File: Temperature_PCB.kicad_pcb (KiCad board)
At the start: 2 copper layers, 29 parts, among them K1 HF115F/024-1H3B, Q1 2N7002, U2 LM393, U5 AMS1117-5.0

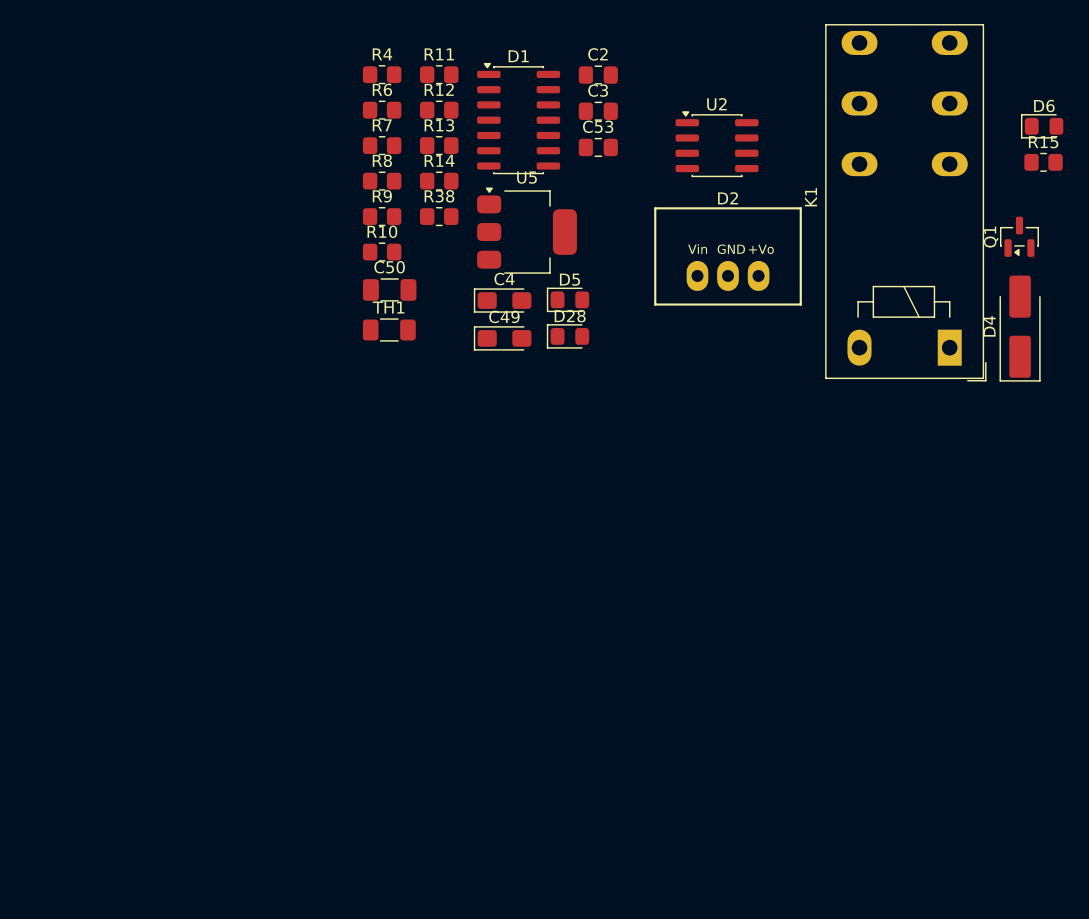
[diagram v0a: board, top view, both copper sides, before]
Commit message: VER1.0: плата разведена, файлы для производства готовы
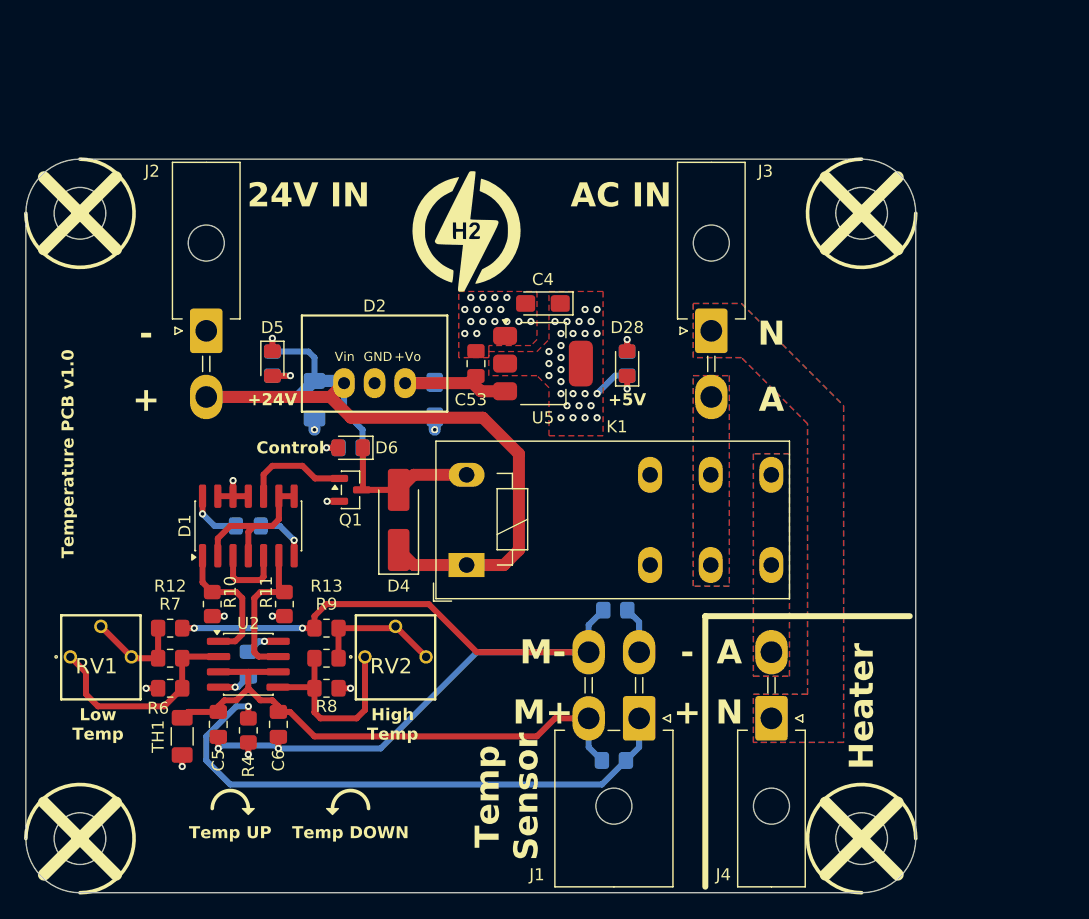
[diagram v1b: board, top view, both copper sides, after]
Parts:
- added C5: 100n, Capacitor_SMD:C_0805_2012Metric_Pad1.18x1.45mm_HandSolder, F.Cu at (127.5, 141.5)
- added C6: 100n, Capacitor_SMD:C_0805_2012Metric_Pad1.18x1.45mm_HandSolder, F.Cu at (132.5, 141.5)
- added D3: Logo, Logo_My:Logo_Company_2, F.Cu at (148.1, 100.5)
- added H1: MountingHole, MountingHole:MountingHole_4.3mm_M4, F.Cu at (181.0, 99.0)
- added H2: MountingHole, MountingHole:MountingHole_4.3mm_M4, F.Cu at (116.0, 99.0)
- added H3: MountingHole, MountingHole:MountingHole_4.3mm_M4, F.Cu at (181.0, 151.0)
- added H4: MountingHole, MountingHole:MountingHole_4.3mm_M4, F.Cu at (116.0, 151.0)
- added J1: ~, Connector_Molex:Molex_Mini-Fit_Jr_5569-04A2_2x02_P4.20mm_Horizontal, F.Cu at (162.5, 141.0)
- added J2: ~, Connector_Molex:Molex_Mini-Fit_Jr_5569-02A2_2x01_P4.20mm_Horizontal, F.Cu at (126.5, 108.8)
- added J3: ~, Connector_Molex:Molex_Mini-Fit_Jr_5569-02A2_2x01_P4.20mm_Horizontal, F.Cu at (168.5, 108.8)
- added J4: ~, Connector_Molex:Molex_Mini-Fit_Jr_5569-02A2_2x01_P4.20mm_Horizontal, F.Cu at (173.5, 141.0)
- added R16: 0, Resistor_SMD:R_0805_2012Metric_Pad1.20x1.40mm_HandSolder, B.Cu at (160.5, 132.0)
- added R5: 0, Resistor_SMD:R_0805_2012Metric_Pad1.20x1.40mm_HandSolder, B.Cu at (160.4, 144.5)
- added RV1: ~, Potentiometer_my:3362P_1, F.Cu at (117.7, 139.4)
- added RV2: ~, Potentiometer_my:3362P_1, F.Cu at (142.2, 139.4)
- C2, C3, C49, C50, R14, R15, R38: moved to B.Cu
- D1: value CD4011 -> ~
- D2: value K7809-500R3 -> ~
- D4: value 1N4007[M7] -> ~
- K1: value HF115F/024-1H3B -> ~
- Q1: value 2N7002 -> ~
- R7: value 20 -> 49.9
- R9: value 49.9 -> 330
- TH1: value Thermistor_NTC_3Wire -> Thermistor_NTC
- U2: value LM393 -> ~
- U5: value AMS1117-5.0 -> ~
- moved D6 63.6 mm to (138.5, 118.5), turned to 180 degrees
- moved R15 62.3 mm to (138.5, 118.5)
- moved Q1 59.5 mm to (138.5, 122.0), turned to 0 degrees
- moved U2 58.1 mm to (130.0, 136.5)
- moved C2 57.0 mm to (130.0, 136.5), turned to -90 degrees
- moved R4 55.6 mm to (130.0, 142.0), turned to -90 degrees
- moved D4 54.1 mm to (142.5, 124.5)
- moved R6 51.2 mm to (123.5, 138.5), turned to 180 degrees
- moved R12 48.5 mm to (123.5, 133.5), turned to 180 degrees
- moved R7 46.1 mm to (123.5, 136.0)
- moved R11 45.9 mm to (133.0, 131.5), turned to -90 degrees
- moved C3 45.1 mm to (130.0, 125.0)
- moved K1 44.1 mm to (148.2, 128.2), turned to 0 degrees
- moved R8 42.4 mm to (136.5, 138.5)
- moved R13 41.2 mm to (136.5, 133.5)
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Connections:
- K1 pad 11: unconnected-(K1-Pad11) -> /A_IN
- K1 pad 12: unconnected-(K1-Pad12) -> (no net)
- K1 pad 14: unconnected-(K1-Pad14) -> /A_OUT
- K1 pad 21: (no net) -> /A_IN
- K1 pad 24: (no net) -> /A_OUT
- R12 pad 1: GND -> Net-(J1-Pin_4)
- R13 pad 1: GND -> Net-(J1-Pin_4)
- R4 pad 1: Net-(J1-Pin_2) -> Net-(J1-Pin_1)
- TH1 pad 2: Net-(J1-Pin_2) -> GND
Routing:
- net Net-(J1-Pin_4): track 0.00 -> 77.1 mm, vias 0 -> 4
- net +24V: track 0.00 -> 72.4 mm
- net Net-(J1-Pin_1): track 0.00 -> 48.0 mm, vias 0 -> 1
- net Net-(J1-Pin_2): track 0.00 -> 47.9 mm
- net GND: track 0.00 -> 21.2 mm, vias 0 -> 25
- net Net-(U2A--): track 0.00 -> 18.3 mm
- net Net-(U2B-+): track 0.00 -> 16.7 mm
- net +5V: track 0.00 -> 15.6 mm, vias 0 -> 35
- net Net-(D1-B): track 0.00 -> 13.1 mm
- net Net-(D4-A): track 0.00 -> 12.8 mm
- net Net-(D1-D): track 0.00 -> 12.5 mm
- net /+9V: track 0.00 -> 11.8 mm
- net Net-(D1-A): track 0.00 -> 11.3 mm
- net Net-(R13-Pad2): track 0.00 -> 10.9 mm
- net /Control: track 0.00 -> 8.82 mm
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- added copper zone on F.Cu, net +5V
- added copper zone on In2.Cu, net +5V
- added copper zone on B.Cu, net /A_IN
- added copper zone on F.Cu, net /A_IN
- added copper zone on B.Cu, net /A_OUT
- added copper zone on F.Cu, net /A_OUT
- added copper zone on B.Cu, net /N
- added copper zone on F.Cu, net /N
- added copper zone on F.Cu, net GND
- added copper zone on In1.Cu, net GND
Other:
- board outline added: 74 x 61 mm
- copper layers 2 -> 4
- board text added: "+"
- board text added: "+24V"
- board text added: "+5V"
- board text added: "-"
- board text added: "24V IN"
- board text added: "A"
- board text added: "AC IN"
- board text added: "Control"
- board text added: "GND"
- board text added: "Heater"
- board text added: "High Temp"
- board text added: "Low Temp"
- board text added: "M+"
- board text added: "M-"
- board text added: "N"
- board text added: "Temp DOWN"
- board text added: "Temp Sensor"
- board text added: "Temp UP"
- board text added: "Temperature PCB v1.0"
